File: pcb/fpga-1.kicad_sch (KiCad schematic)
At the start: 1 part, among them U7 XC7A100T-FGG484

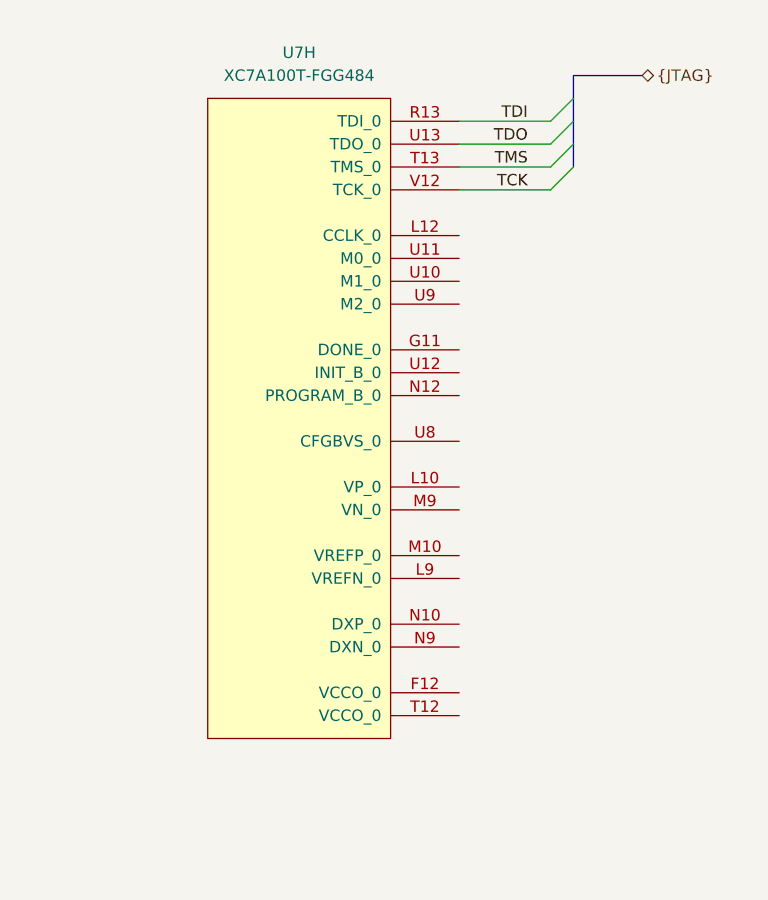
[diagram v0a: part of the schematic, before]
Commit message: jtag, dcplng
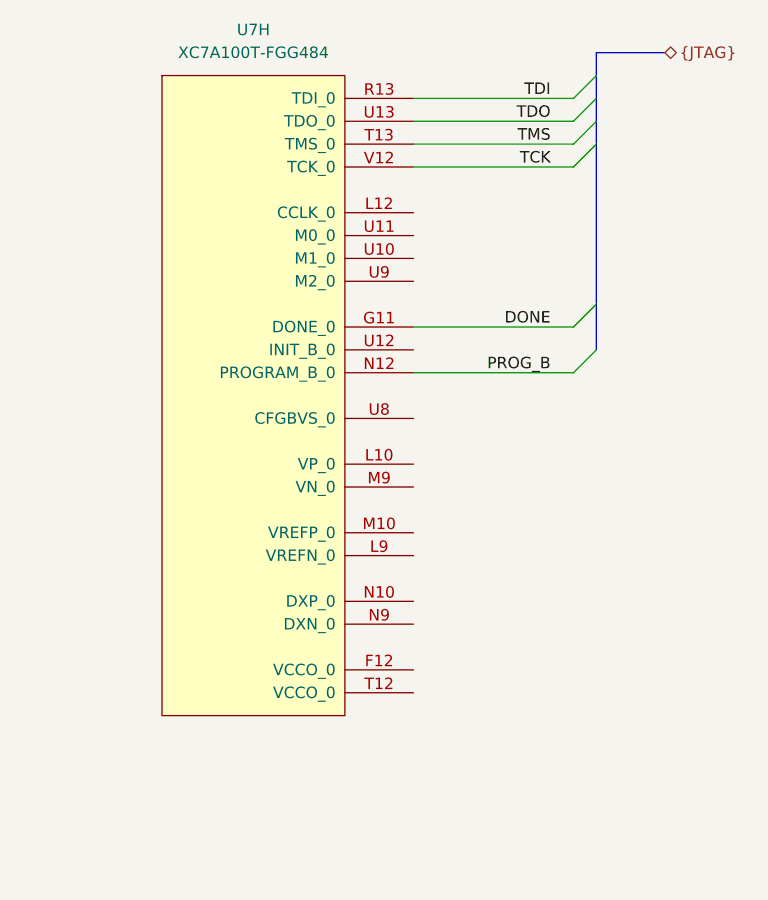
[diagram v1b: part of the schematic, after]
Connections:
- net DONE: now reaches U7.G11 (DONE_0)
- net PROG_B: now reaches U7.N12 (PROGRAM_B_0)
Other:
- moved on the sheet: U7H
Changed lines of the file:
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@@
 	)
 	(bus_entry
-		(at 256.54 38.1)
+		(at 259.08 53.34)
 		(size 2.54 -2.54)
 		(stroke
@@
 	)
 	(bus_entry
-		(at 256.54 33.02)
+		(at 259.08 35.56)
 		(size 2.54 -2.54)
 		(stroke
@@
 	)
 	(bus_entry
-		(at 256.54 30.48)
+		(at 259.08 30.48)
 		(size 2.54 -2.54)
 		(stroke
@@
 	)
 	(bus_entry
-		(at 256.54 35.56)
+		(at 259.08 58.42)
+		(size 2.54 -2.54)
+		(stroke
+			(width 0)
+			(type default)
+		)
+	)
+	(bus_entry
+		(at 259.08 27.94)
+		(size 2.54 -2.54)
+		(stroke
+			(width 0)
+			(type default)
+		)
+	)
+	(bus_entry
+		(at 259.08 33.02)
 		(size 2.54 -2.54)
 		(stroke
@@
 	(wire
 		(pts
-			(xy 246.38 30.48) (xy 256.54 30.48)
+			(xy 241.3 30.48) (xy 259.08 30.48)
+		)
+		(stroke
+			(width 0)
+			(type default)
+		)
+	)
+	(wire
+		(pts
+			(xy 241.3 27.94) (xy 259.08 27.94)
 		)
 		(stroke
@@
 	(bus
 		(pts
-			(xy 259.08 35.56) (xy 259.08 33.02)
+			(xy 261.62 33.02) (xy 261.62 30.48)
 		)
 		(stroke
@@
 	(wire
 		(pts
-			(xy 246.38 33.02) (xy 256.54 33.02)
+			(xy 241.3 58.42) (xy 259.08 58.42)
+		)
+		(stroke
+			(width 0)
+			(type default)
+		)
+	)
+	(wire
+		(pts
+			(xy 241.3 33.02) (xy 259.08 33.02)
 		)
 		(stroke
@@
 	(bus
 		(pts
-			(xy 259.08 30.48) (xy 259.08 27.94)
+			(xy 261.62 27.94) (xy 261.62 25.4)
 		)
 		(stroke
@@
 	(bus
 		(pts
-			(xy 259.08 25.4) (xy 266.7 25.4)
+			(xy 261.62 22.86) (xy 269.24 22.86)
+		)
+		(stroke
+			(width 0)
+			(type default)
+		)
+	)
+	(bus
+		(pts
+			(xy 261.62 50.8) (xy 261.62 55.88)
 		)
 		(stroke
@@
 	(wire
 		(pts
-			(xy 246.38 35.56) (xy 256.54 35.56)
+			(xy 241.3 53.34) (xy 259.08 53.34)
 		)
 		(stroke
@@
 	(bus
 		(pts
-			(xy 259.08 33.02) (xy 259.08 30.48)
+			(xy 261.62 30.48) (xy 261.62 27.94)
 		)
 		(stroke
@@
 	(wire
 		(pts
-			(xy 246.38 38.1) (xy 256.54 38.1)
+			(xy 241.3 35.56) (xy 259.08 35.56)
 		)
 		(stroke
@@
 	(bus
 		(pts
-			(xy 259.08 27.94) (xy 259.08 25.4)
+			(xy 261.62 25.4) (xy 261.62 22.86)
+		)
+		(stroke
+			(width 0)
+			(type default)
+		)
+	)
+	(bus
+		(pts
+			(xy 261.62 33.02) (xy 261.62 50.8)
 		)
 		(stroke
@@
 	)
 	(label "TDO"
-		(at 254 33.02 180)
+		(at 256.54 30.48 180)
 		(effects
 			(font
@@
 	)
 	(label "TCK"
-		(at 254 38.1 180)
+		(at 256.54 35.56 180)
 		(effects
 			(font
@@
 	)
 	(label "TMS"
-		(at 254 35.56 180)
+		(at 256.54 33.02 180)
 		(effects
 			(font
@@
 		)
 	)
-	(label "TDI"
-		(at 254 30.48 180)
+	(label "DONE"
+		(at 256.54 53.34 180)
 		(effects
 			(font
@@
 		)
 	)
+	(label "TDI"
+		(at 256.54 27.94 180)
+		(effects
+			(font
+				(size 1.27 1.27)
+			)
+			(justify right bottom)
+		)
+	)
+	(label "PROG_B"
+		(at 256.54 58.42 180)
+		(effects
+			(font
+				(size 1.27 1.27)
+			)
+			(justify right bottom)
+		)
+	)
 	(hierarchical_label "{JTAG}"
 		(shape bidirectional)
-		(at 266.7 25.4 0)
+		(at 269.24 22.86 0)
 		(effects
 			(font
@@
 	(symbol
 		(lib_id "library:XC7A100T-FGG484")
-		(at 228.6 81.28 0)
+		(at 223.52 78.74 0)
 		(unit 8)
 		(exclude_from_sim no)
@@
 		(fields_autoplaced yes)
 		(property "Reference" "U7"
-			(at 228.6 22.86 0)
+			(at 223.52 20.32 0)
 			(effects
 				(font
@@
 		)
 		(property "Value" "XC7A100T-FGG484"
-			(at 228.6 25.4 0)
+			(at 223.52 22.86 0)
 			(effects
 				(font
@@
 		)
 		(property "Footprint" "library:Xilinx_FGG484"
-			(at 228.6 81.28 0)
+			(at 223.52 78.74 0)
 			(effects
 				(font
@@
 		)
 		(property "Datasheet" ""
-			(at 228.6 81.28 0)
+			(at 223.52 78.74 0)
 			(effects
 				(font
@@
 		)
 		(property "Description" "Artix 7 T 100 XC7A100T-FGG484"
-			(at 228.6 193.04 0)
+			(at 223.52 190.5 0)
 			(effects
 				(font
@@
 		)
 		(property "Name" ""
-			(at 228.6 81.28 0)
+			(at 223.52 78.74 0)
 			(effects
 				(font
